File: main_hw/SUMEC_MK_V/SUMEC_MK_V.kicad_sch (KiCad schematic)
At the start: 10 parts

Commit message: 67yfhtgftu
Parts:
- renumbered TP19 to TP1, TP22 to TP10, TP1 to TP2, TP2 to TP3, TP3 to TP4, TP4 to TP5, TP5 to TP6, TP6 to TP7, TP20 to TP8, TP21 to TP9
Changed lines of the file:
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@@
 		(dnp no)
 		(fields_autoplaced yes)
-		(property "Reference" "TP20"
+		(property "Reference" "TP8"
 			(at 165.1 184.6579 0)
 			(effects
@@
 			(project "SUMEC_MK_V"
 				(path "/900bd7ac-cdf9-4a2f-8b1f-2c21e3760046"
-					(reference "TP20")
+					(reference "TP8")
 					(unit 1)
 				)
@@
 		(dnp no)
 		(fields_autoplaced yes)
-		(property "Reference" "TP4"
+		(property "Reference" "TP5"
 			(at 153.67 184.6579 0)
 			(effects
@@
 			(project "SUMEC_MK_V"
 				(path "/900bd7ac-cdf9-4a2f-8b1f-2c21e3760046"
-					(reference "TP4")
+					(reference "TP5")
 					(unit 1)
 				)
@@
 		(dnp no)
 		(fields_autoplaced yes)
-		(property "Reference" "TP3"
+		(property "Reference" "TP4"
 			(at 149.86 184.6579 0)
 			(effects
@@
 			(project "SUMEC_MK_V"
 				(path "/900bd7ac-cdf9-4a2f-8b1f-2c21e3760046"
-					(reference "TP3")
+					(reference "TP4")
 					(unit 1)
 				)
@@
 		(dnp no)
 		(fields_autoplaced yes)
-		(property "Reference" "TP22"
+		(property "Reference" "TP10"
 			(at 172.72 184.6579 0)
 			(effects
@@
 			(project "SUMEC_MK_V"
 				(path "/900bd7ac-cdf9-4a2f-8b1f-2c21e3760046"
-					(reference "TP22")
+					(reference "TP10")
 					(unit 1)
 				)
@@
 		(dnp no)
 		(fields_autoplaced yes)
-		(property "Reference" "TP21"
+		(property "Reference" "TP9"
 			(at 168.91 184.6579 0)
 			(effects
@@
 			(project "SUMEC_MK_V"
 				(path "/900bd7ac-cdf9-4a2f-8b1f-2c21e3760046"
-					(reference "TP21")
+					(reference "TP9")
 					(unit 1)
 				)
@@
 		(dnp no)
 		(fields_autoplaced yes)
-		(property "Reference" "TP5"
+		(property "Reference" "TP6"
 			(at 157.48 184.6579 0)
 			(effects
@@
 			(project "SUMEC_MK_V"
 				(path "/900bd7ac-cdf9-4a2f-8b1f-2c21e3760046"
-					(reference "TP5")
+					(reference "TP6")
 					(unit 1)
 				)
@@
 		(dnp no)
 		(fields_autoplaced yes)
-		(property "Reference" "TP6"
+		(property "Reference" "TP7"
 			(at 161.29 184.6579 0)
 			(effects
@@
 			(project "SUMEC_MK_V"
 				(path "/900bd7ac-cdf9-4a2f-8b1f-2c21e3760046"
-					(reference "TP6")
+					(reference "TP7")
 					(unit 1)
 				)
@@
 		(dnp no)
 		(fields_autoplaced yes)
-		(property "Reference" "TP19"
+		(property "Reference" "TP1"
 			(at 138.43 184.6579 0)
 			(effects
@@
 			(project "SUMEC_MK_V"
 				(path "/900bd7ac-cdf9-4a2f-8b1f-2c21e3760046"
-					(reference "TP19")
+					(reference "TP1")
 					(unit 1)
 				)
@@
 		(dnp no)
 		(fields_autoplaced yes)
-		(property "Reference" "TP1"
+		(property "Reference" "TP2"
 			(at 142.24 184.6579 0)
 			(effects
@@
 			(project "SUMEC_MK_V"
 				(path "/900bd7ac-cdf9-4a2f-8b1f-2c21e3760046"
-					(reference "TP1")
+					(reference "TP2")
 					(unit 1)
 				)
@@
 		(dnp no)
 		(fields_autoplaced yes)
-		(property "Reference" "TP2"
+		(property "Reference" "TP3"
 			(at 146.05 184.6579 0)
 			(effects
@@
 			(project "SUMEC_MK_V"
 				(path "/900bd7ac-cdf9-4a2f-8b1f-2c21e3760046"
-					(reference "TP2")
-					(unit 1)
-				)
+					(reference "TP3")
+					(unit 1)
+				)

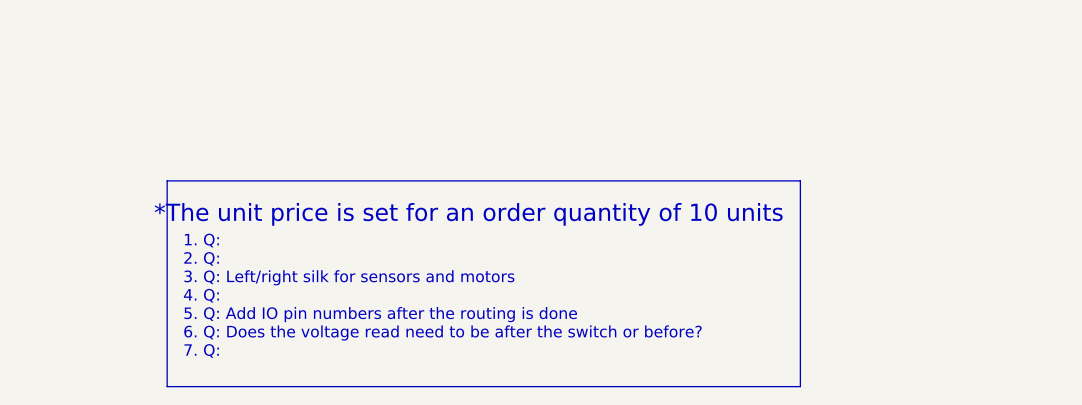
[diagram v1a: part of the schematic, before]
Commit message: MK5 changes and deletion of useless files
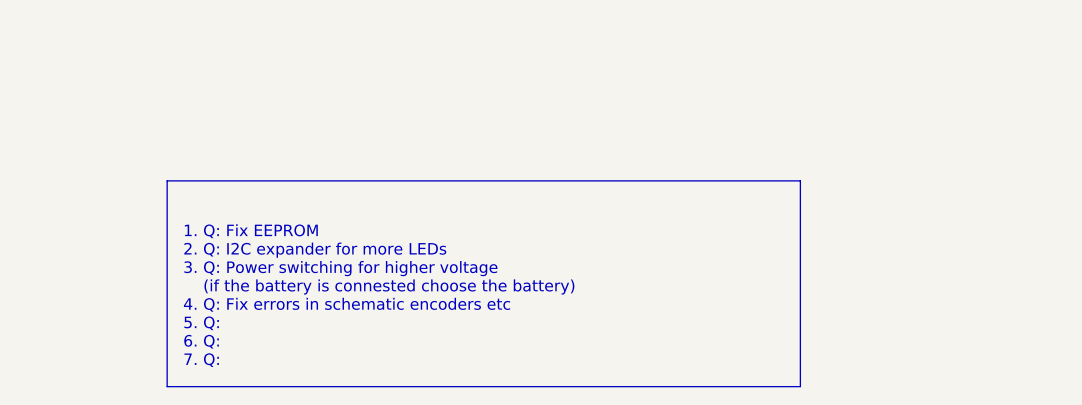
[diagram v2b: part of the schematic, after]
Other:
- note added: "1. Q: Fix EEPROM 2. Q: I2C expander for more LEDs 3. Q: Power switching for higher voltage (if the battery is connested choose the battery) 4. Q: Fix errors in schematic encoders etc 5. Q: 6. Q: 7. Q:"
- note removed: "*The unit price is set for an order quantity of 10 units"
- note removed: "1. Q: 2. Q: 3. Q: Left/right silk for sensors and motors 4. Q: 5. Q: Add IO pin numbers after the routing is done 6. Q: Does the voltage read need to be after the switch or before? 7. Q:"
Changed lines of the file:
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@@
 		)
 	)
-	(text "1. Q: \n2. Q: \n3. Q: Left/right silk for sensors and motors\n4. Q: \n5. Q: Add IO pin numbers after the routing is done\n6. Q: Does the voltage read need to be after the switch or before?\n7. Q: "
+	(text "1. Q: Fix EEPROM\n2. Q: I2C expander for more LEDs\n3. Q: Power switching for higher voltage \n	(if the battery is connested choose the battery)\n4. Q: Fix errors in schematic encoders etc\n5. Q: \n6. Q: \n7. Q: "
 		(exclude_from_sim no)
 		(at 20.32 183.134 0)
@@
 		)
 	)
-	(text "*The unit price is set for an order quantity of 10 units"
-		(exclude_from_sim no)
-		(at 52.07 173.99 0)
-		(effects
-			(font
-				(face "Bahnschrift")
-				(size 1.905 1.905)
-				(color 255 0 0 1)
-			)
-		)
-	)
